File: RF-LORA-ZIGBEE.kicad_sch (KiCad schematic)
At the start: 41 parts, among them J9 LoRa_Anten, Q1 BC847, U10 MASWSS0192, U6 SX1278, Y4 32MHz

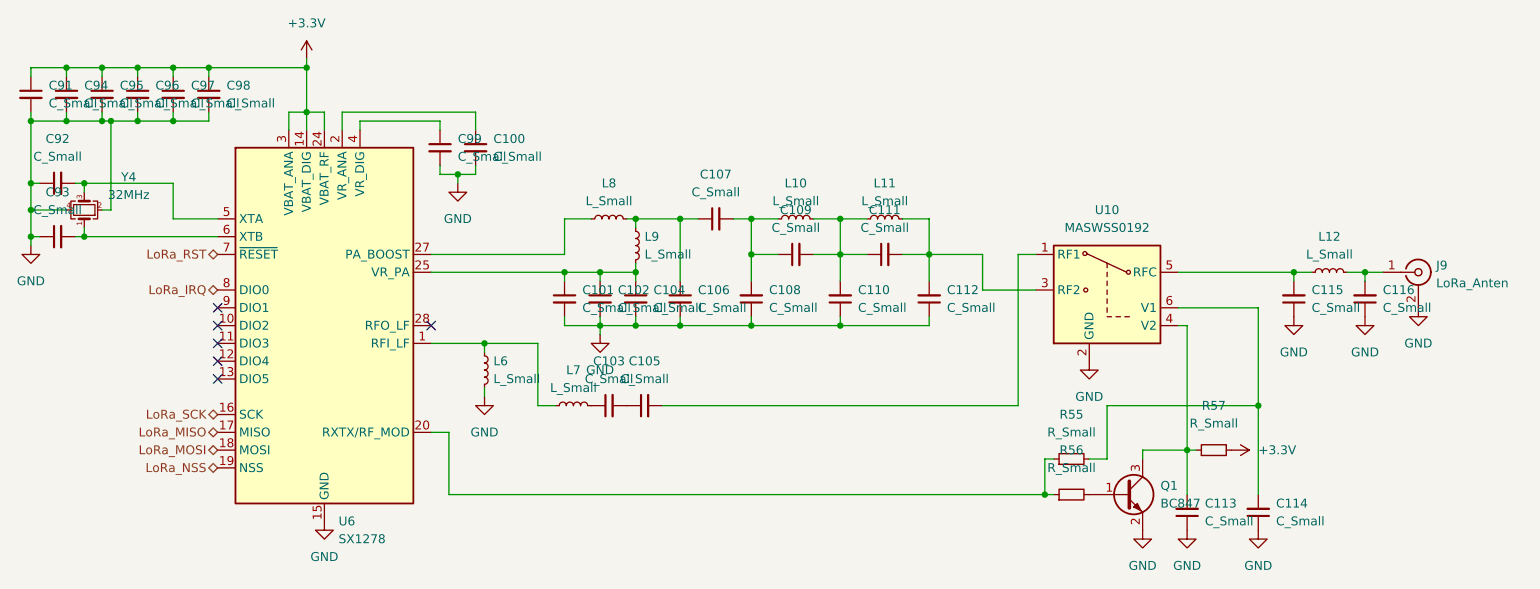
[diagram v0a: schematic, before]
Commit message: Only 1 wire to complete.
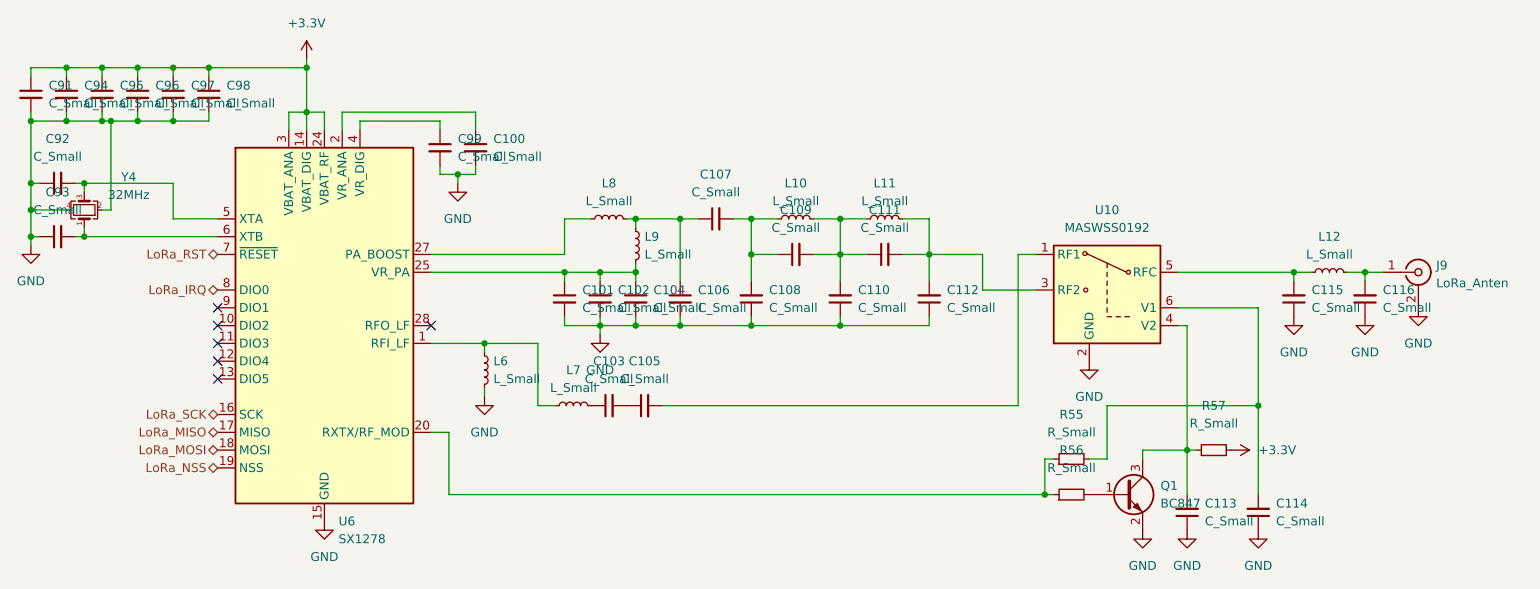
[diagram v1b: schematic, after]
